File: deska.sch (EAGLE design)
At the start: 17 parts, among them Q1 BC547, Q2 BC547

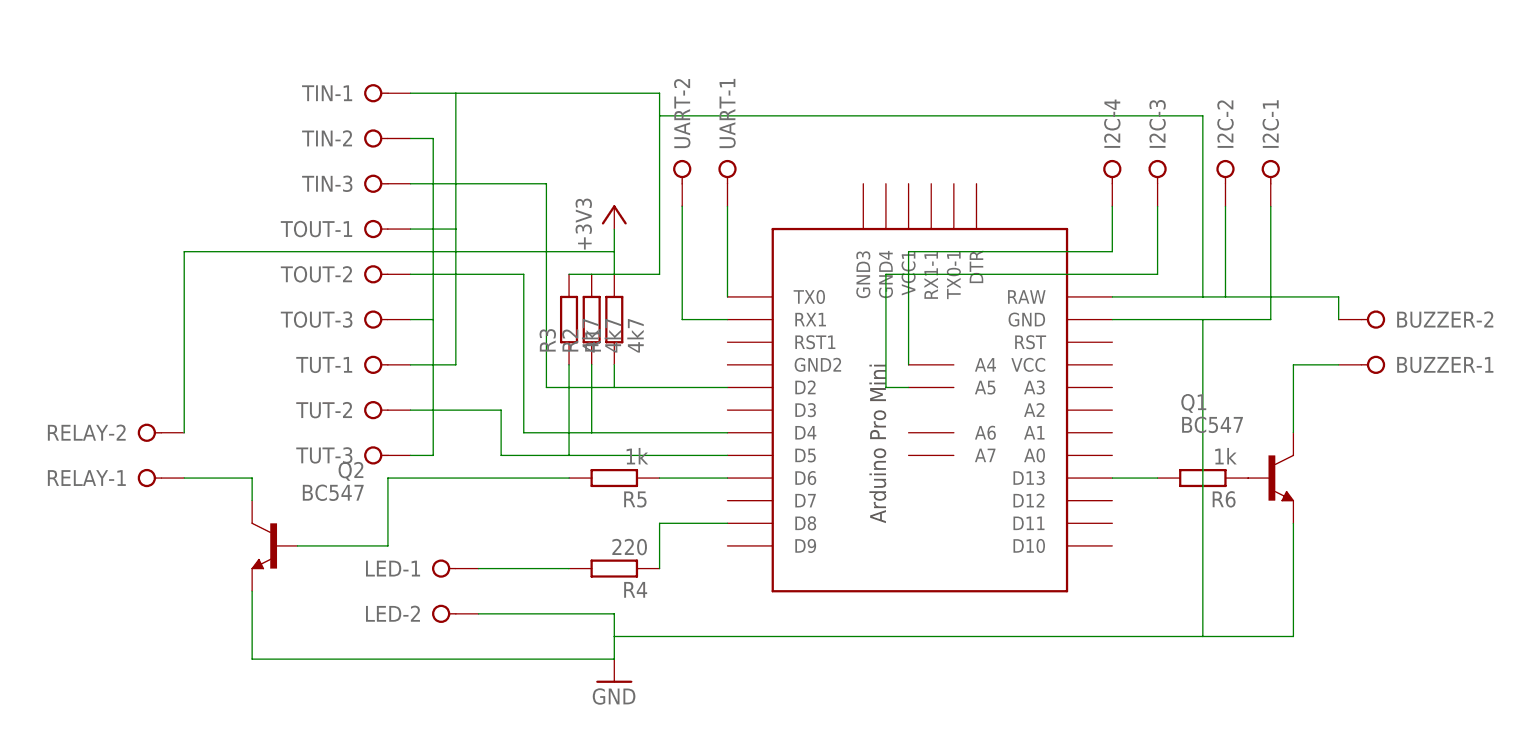
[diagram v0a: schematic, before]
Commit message: +
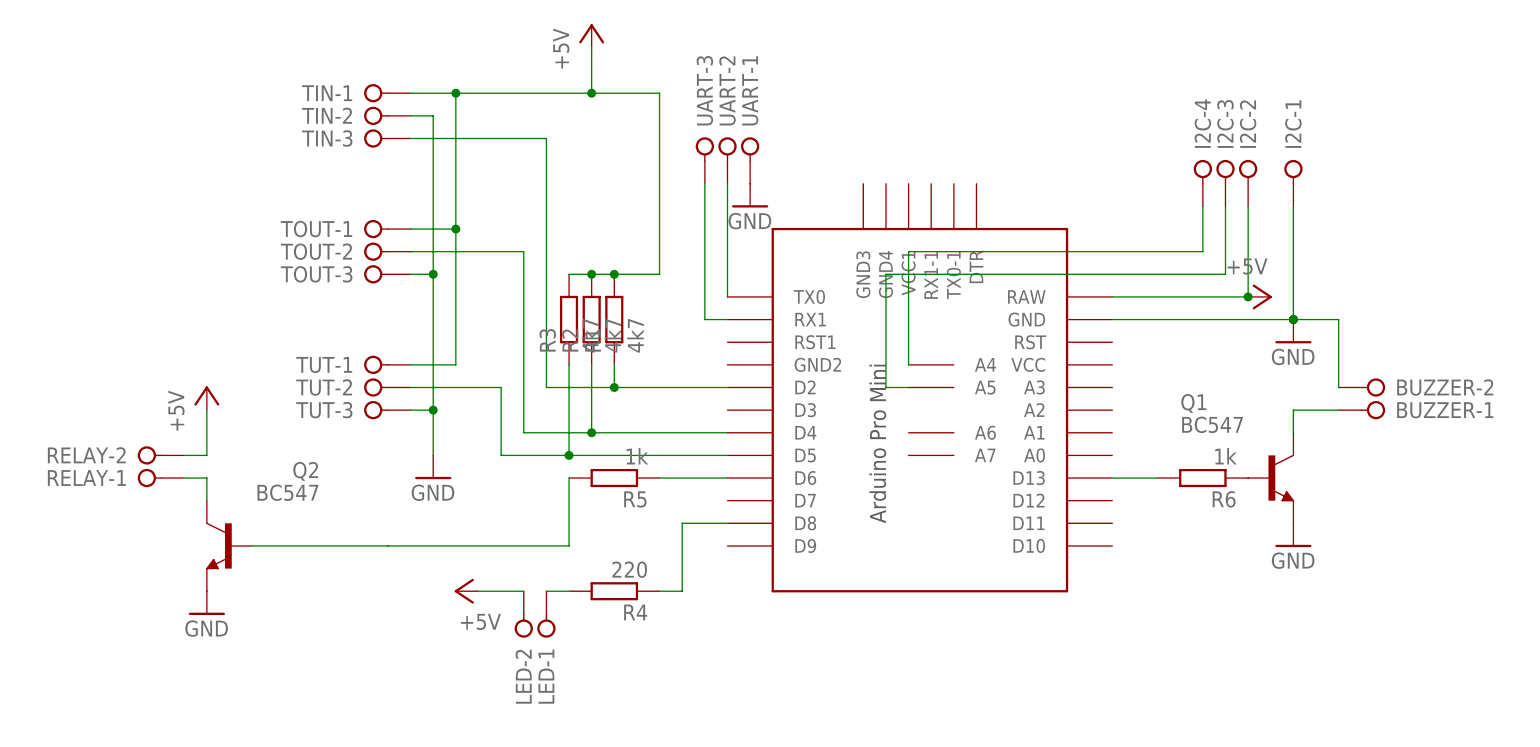
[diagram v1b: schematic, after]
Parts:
- UART: device con-wago-508:W237-02P -> con-wago-508:W237-3E
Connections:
- removed net +3V3: BUZZER-2.KL, I2C-2.KL, R1.2, R2.2, R3.2, RELAY-2.KL, TIN-1.KL, TOUT-1.KL, TUT-1.KL, U$1.RAW
- removed net N$8: TIN-2.KL, TOUT-3.KL, TUT-3.KL
- new net +5V: I2C-2.KL, LED-2.KL, R1.2, R2.2, R3.2, RELAY-2.KL, TIN-1.KL, TOUT-1.KL, TUT-1.KL, U$1.RAW
- net GND: now also BUZZER-2.KL, TIN-2.KL, TOUT-3.KL, TUT-3.KL, UART-1.KL; no longer LED-2.KL
- net N$10: now also UART-3.KL; no longer UART-2.KL
- net N$9: now also UART-2.KL; no longer UART-1.KL
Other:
- moved on the sheet: BUZZER-1, BUZZER-2, I2C-1, I2C-2, I2C-3, I2C-4, LED-1, LED-2, Q2, R4, RELAY-2, TIN-2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
